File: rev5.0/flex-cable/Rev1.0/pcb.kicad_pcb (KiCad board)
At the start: 2 copper layers, 12.5 x 40.6 mm, 2 parts, among them J1 fpc, J2 oled

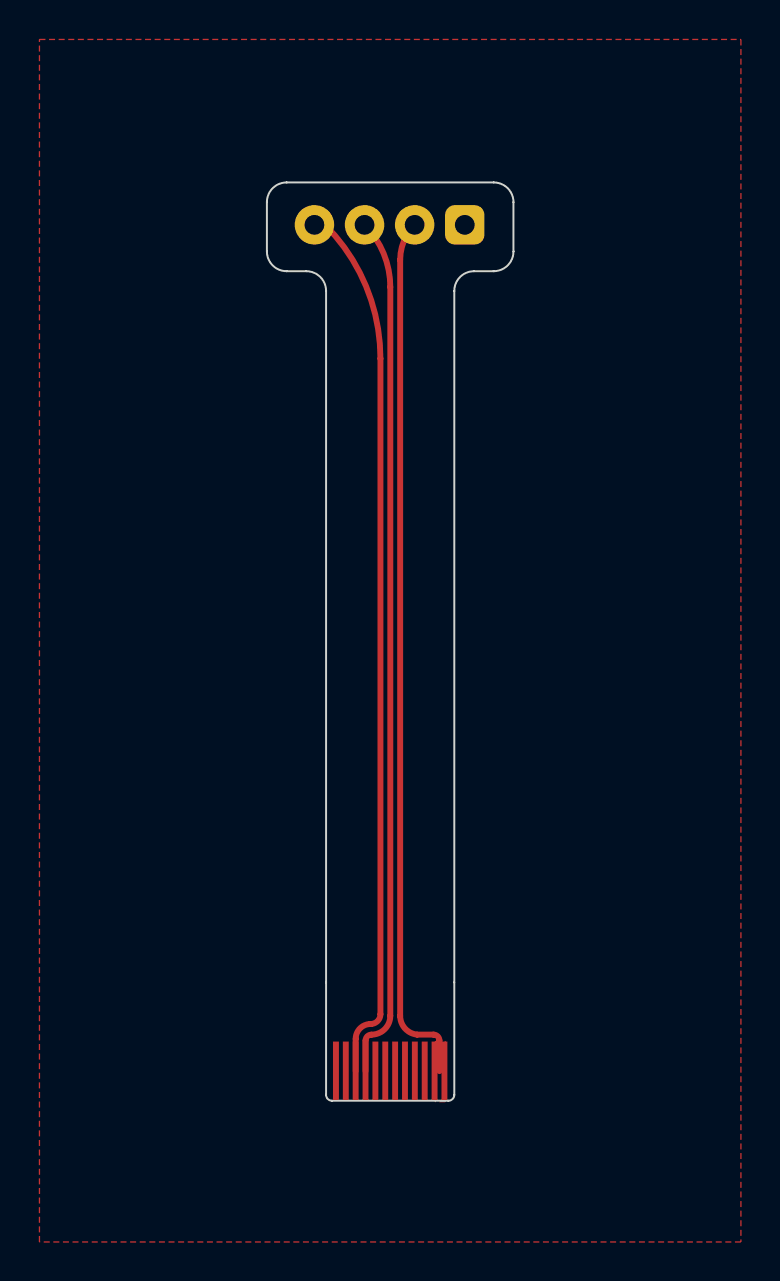
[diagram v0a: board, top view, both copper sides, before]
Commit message: fix some minor issues
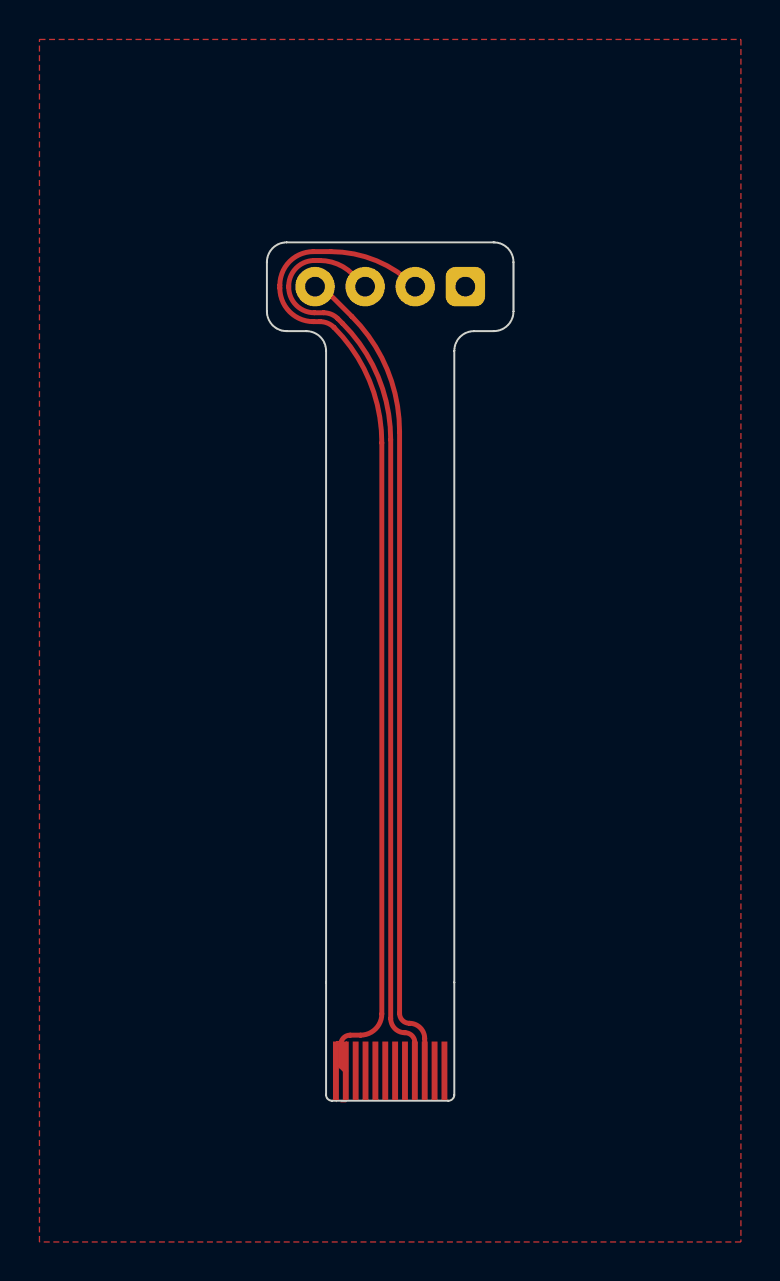
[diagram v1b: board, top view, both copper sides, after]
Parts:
- moved J2 3.13 mm to (136.1, 58.2)
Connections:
- J1 pad 1: GND -> VCC
- J1 pad 10: /misc -> /i2c_sda
- J1 pad 11: VCC -> GND
- J1 pad 12: VCC -> GND
- J1 pad 2: GND -> VCC
- J1 pad 3: /i2c_sda -> /misc
- J1 pad 4: /i2c_scl -> /spi_rst
- J1 pad 5: /spi_cs -> /spi_sdi
- J1 pad 6: /spi_dc -> /spi_sdo
- J1 pad 7: /spi_sdo -> /spi_dc
- J1 pad 8: /spi_sdi -> /spi_cs
- J1 pad 9: /spi_rst -> /i2c_scl
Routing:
- net VCC: track 44.5 -> 51.8 mm
- net /i2c_scl: track 43.9 -> 47.8 mm
- net /i2c_sda: track 44.8 -> 42.0 mm
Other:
- board size 12.5 x 40.6 mm -> 6.5 x 32 mm
